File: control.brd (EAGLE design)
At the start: 165 x 34 mm, 65 parts, among them IC3 ATTINY85-20S

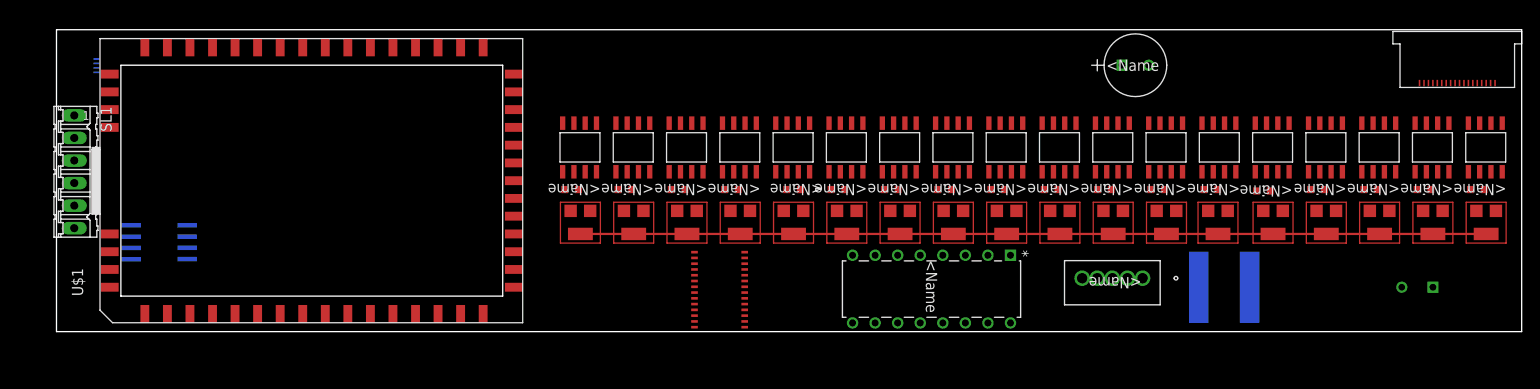
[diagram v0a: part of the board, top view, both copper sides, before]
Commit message: FAIL compact layout
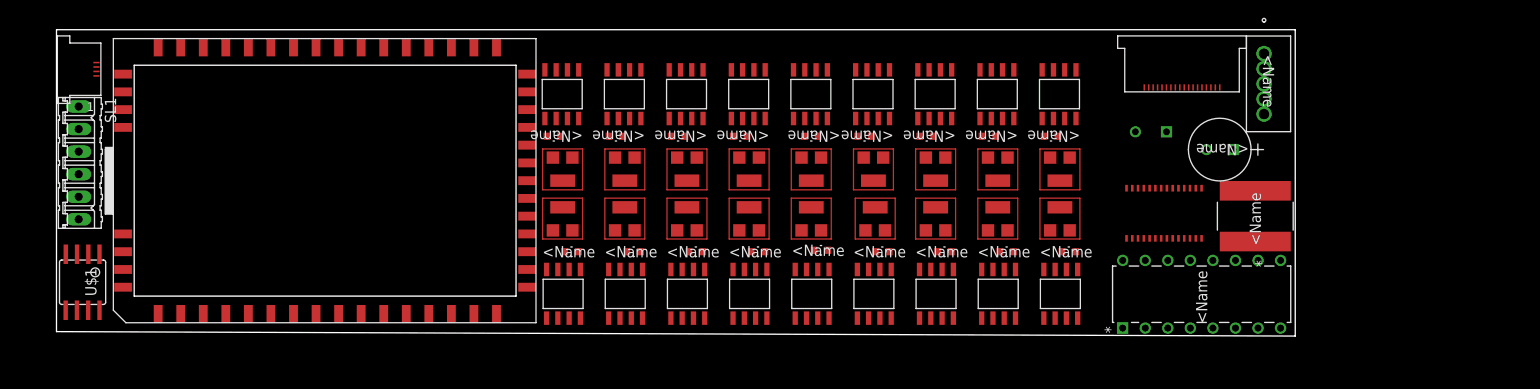
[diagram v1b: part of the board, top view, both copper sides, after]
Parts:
- moved U$18 104.0 mm to (57.0, 14.0), turned to 180 degrees
- moved R8 102.2 mm to (58.0, 9.00), turned to 0 degrees
- moved U$17 100.6 mm to (59.0, 7.00), turned to 180 degrees
- moved U$4 91.0 mm to (64.0, 14.0), turned to 180 degrees
- moved R1 89.3 mm to (65.0, 9.00), turned to 0 degrees
- moved U$3 87.7 mm to (66.0, 7.00), turned to 180 degrees
- moved U$6 78.1 mm to (71.0, 14.0), turned to 180 degrees
- moved R2 76.3 mm to (72.0, 9.00), turned to 0 degrees
- moved U$5 74.8 mm to (73.0, 7.00), turned to 180 degrees
- moved U$8 65.1 mm to (78.0, 14.0), turned to 180 degrees
- moved R3 63.4 mm to (79.0, 9.00), turned to 0 degrees
- moved U$7 62.0 mm to (80.0, 7.00), turned to 180 degrees
- moved U$14 52.1 mm to (85.0, 14.0), turned to 180 degrees
- moved R6 50.3 mm to (86.1, 9.16), turned to 0 degrees
- moved U$13 49.2 mm to (87.0, 7.00), turned to 180 degrees
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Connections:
- removed net B0: IC3.5, SL1.5
- removed net B1: IC3.6, SL1.6
- removed net B2: IC3.7
- removed net N$39: SL1.3
- new net ENC1: IC3.6, SL1.5
- new net ENC2: IC3.7, SL1.6
- new net ENCOUT: IC3.5, U$1.USB1_N
- net 3V3: now also SL1.3
- net LEDSTR_1: now also U$44.P$9; no longer U$44.P$1
- net LEDSTR_11: now also U$44.P$1; no longer U$44.P$9
- net LEDSTR_2: now also U$44.P$8; no longer U$44.P$2
- net LEDSTR_3: now also U$44.P$7; no longer U$44.P$3
- net LEDSTR_4: now also U$44.P$6; no longer U$44.P$4
- net LEDSTR_5: now also U$44.P$3; no longer U$44.P$7
- net LEDSTR_6: now also U$44.P$4; no longer U$44.P$6
- net LEDSTR_8: now also U$44.P$2; no longer U$44.P$8
- net ZN0: now also U$37.P$13; no longer U$37.P$6
- net ZN1: now also U$37.P$12; no longer U$37.P$7
- net ZN2: now also U$37.P$11; no longer U$37.P$8
- net ZN3: now also U$37.P$10; no longer U$37.P$9
- net ZN4: now also U$37.P$9; no longer U$37.P$10
- net ZN5: now also U$37.P$8; no longer U$37.P$11
- net ZN6: now also U$37.P$7; no longer U$37.P$12
- net ZN7: now also U$37.P$6; no longer U$37.P$13
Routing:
- net GND: track 103.0 -> 0.00 mm
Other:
- board size 165 x 34 mm -> 139.5 x 34.5 mm

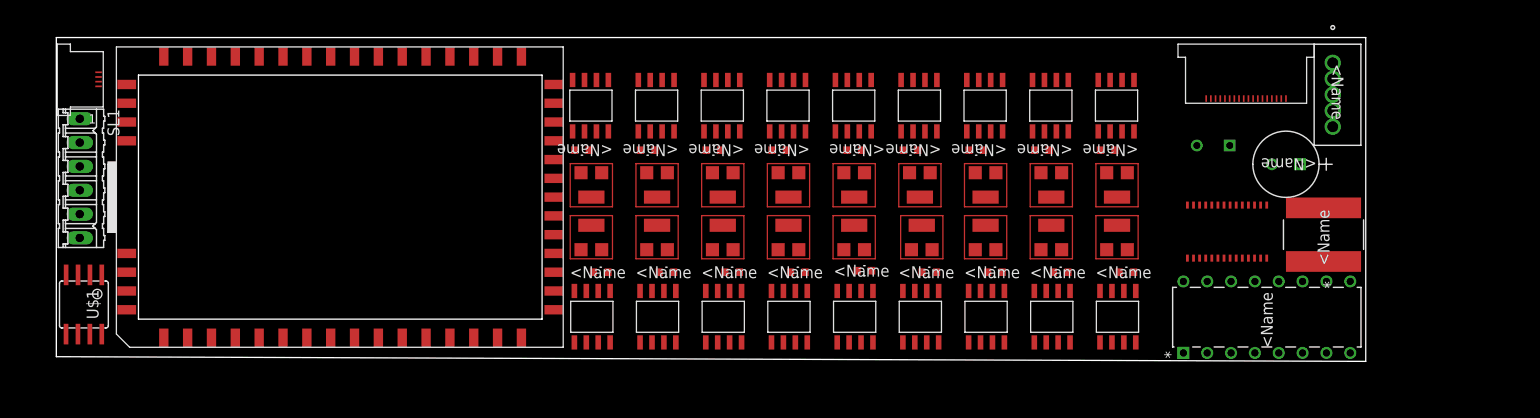
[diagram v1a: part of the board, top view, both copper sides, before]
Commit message: completes first ideration
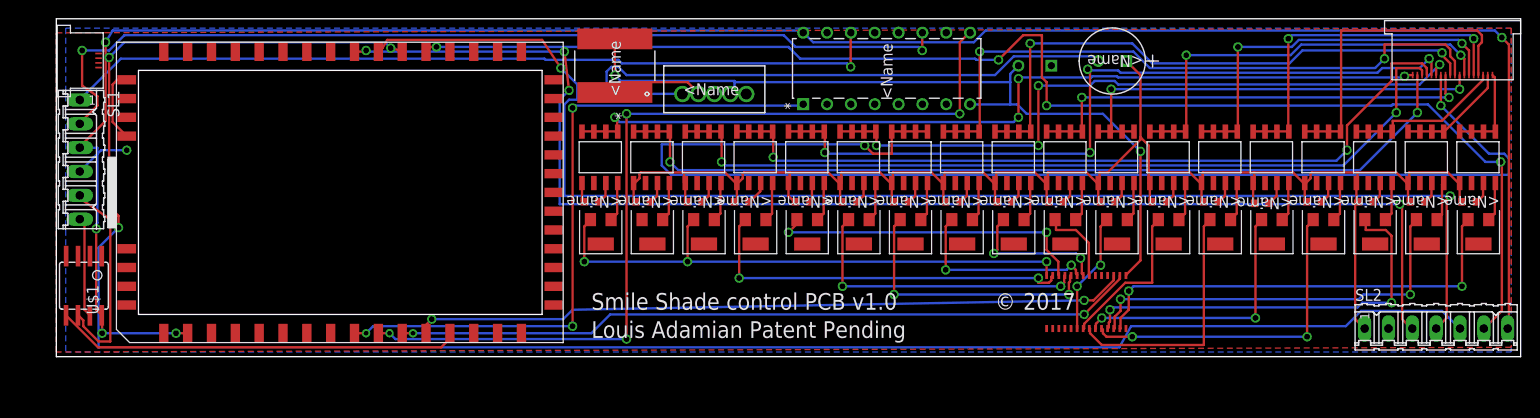
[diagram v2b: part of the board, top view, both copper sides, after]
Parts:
- removed U$43: 2N7002P, LED Driver:SOT23
- added SL2: (no value), con-amp-quick:07P
- added U$38: 2N7002P, Smile_Shade:SOT23
- U$10, U$12, U$14, U$16, U$18, U$20, U$22, U$24, U$26, U$28, U$30, U$32, U$34, U$4, U$41, U$6, U$8: device LED Driver:SOT23 -> Smile_Shade:SOT23
- moved R8 92.8 mm to (150.5, 16.5), turned to 180 degrees
- moved U$17 91.2 mm to (149.5, 18.5), turned to 0 degrees
- moved U$4 82.0 mm to (146.0, 12.0), turned to 0 degrees
- moved R1 80.4 mm to (145.0, 16.5), turned to 180 degrees
- moved U$3 78.8 mm to (144.0, 18.5), turned to 0 degrees
- moved U$36 77.6 mm to (59.5, 31.0)
- moved U$6 69.5 mm to (140.5, 12.0), turned to 0 degrees
- moved R2 67.9 mm to (139.5, 16.5), turned to 180 degrees
- moved U$5 66.5 mm to (138.5, 18.5), turned to 0 degrees
- moved U$35 63.7 mm to (73.5, 29.0), turned to 0 degrees
- moved U$8 57.0 mm to (135.0, 12.0), turned to 0 degrees
- moved R3 55.5 mm to (134.0, 16.5), turned to 180 degrees
- moved U$7 54.2 mm to (133.0, 18.5), turned to 0 degrees
- moved U$2 48.4 mm to (97.3, 34.5)
- moved R6 42.9 mm to (128.4, 16.3), turned to 180 degrees
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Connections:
- removed net 24V: U$2.8
- new net +3V3: IC3.8
- new net ENDSTOP0: SL2.3, U$1.CSID0
- new net ENDSTOP1: SL2.4, U$1.CSID1
- new net ENDSTOP2: SL2.5, U$1.CSID2
- new net ENDSTOP3: SL2.6, U$1.CSID3
- net 3V3: now also SL2.7, U$2.16; no longer IC3.8
- net 48V: now also SL2.1
- net 5V: now also U$2.8; no longer U$2.16
- net ENCOUT: now also U$1.UART2-TX; no longer U$1.USB1_N
- net GND: now also SL2.2, U$38.P$1; no longer U$43.P$1
- net LEDSTR_1: now also U$44.P$1; no longer U$44.P$9
- net LEDSTR_11: now also U$44.P$11; no longer U$44.P$1
- net LEDSTR_2: now also U$44.P$2; no longer U$44.P$8
- net LEDSTR_3: now also U$44.P$3; no longer U$44.P$7
- net LEDSTR_4: now also U$44.P$4; no longer U$44.P$6
- net LEDSTR_5: now also U$44.P$7; no longer U$44.P$3
- net LEDSTR_6: now also U$44.P$6; no longer U$44.P$4
- net LEDSTR_8: now also U$44.P$8; no longer U$44.P$2
- net LEDSTR_9: now also U$44.P$9; no longer U$44.P$11
- net N$11: now also U$12.P$3; no longer U$14.P$3
- net N$13: now also U$10.P$3; no longer U$16.P$3
- net N$15: now also U$38.P$3; no longer U$18.P$3
- net N$17: now also U$18.P$3; no longer U$20.P$3
- net N$19: now also U$20.P$3; no longer U$22.P$3
- net N$21: now also U$22.P$3; no longer U$24.P$3
- net N$23: now also U$24.P$3; no longer U$26.P$3
- net N$25: now also U$32.P$3; no longer U$28.P$3
- net N$29: now also U$28.P$3; no longer U$32.P$3
- net N$31: now also U$26.P$3; no longer U$34.P$3
- net N$35: now also U$34.P$3; no longer U$41.P$3
- net N$37: now also U$41.P$3; no longer U$43.P$3
- net N$7: now also U$16.P$3; no longer U$10.P$3
- net N$9: now also U$14.P$3; no longer U$12.P$3
- net ZN0: now also U$38.P$2; no longer U$18.P$2
- net ZN11: now also U$32.P$2; no longer U$28.P$2
- net ZN12: now also U$24.P$2; no longer U$26.P$2
- net ZN13: now also U$18.P$2; no longer U$20.P$2
- net ZN14: now also U$20.P$2; no longer U$22.P$2
- net ZN15: now also U$22.P$2; no longer U$24.P$2
- net ZN16: now also U$41.P$2; no longer U$43.P$2
- net ZN4: now also U$12.P$2; no longer U$14.P$2
- net ZN5: now also U$14.P$2; no longer U$12.P$2
- net ZN6: now also U$16.P$2; no longer U$10.P$2
- net ZN7: now also U$10.P$2; no longer U$16.P$2
- net ZN8: now also U$26.P$2; no longer U$41.P$2
- net ZN9: now also U$28.P$2; no longer U$32.P$2
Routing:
- net 3V3: track 0.00 -> 225.4 mm, vias 0 -> 5
- net ENDSTOP2: track 0.00 -> 212.2 mm, vias 0 -> 3
- net 48V: track 0.00 -> 175.5 mm
- net ENDSTOP1: track 0.00 -> 146.3 mm, vias 0 -> 2
- net ENDSTOP3: track 0.00 -> 144.8 mm, vias 0 -> 4
- net ENDSTOP0: track 0.00 -> 142.6 mm, vias 0 -> 4
- net LEDSTR_12: track 0.00 -> 138.6 mm, vias 0 -> 2
- net M2B: track 0.00 -> 102.2 mm, vias 0 -> 2
- net LEDSTR_17: track 0.00 -> 95.4 mm, vias 0 -> 4
- net M1: track 0.00 -> 95.3 mm, vias 0 -> 4
- net LEDSTR_18: track 0.00 -> 93.6 mm, vias 0 -> 2
- net LEDSTR_16: track 0.00 -> 89.6 mm, vias 0 -> 2
- net M2A: track 0.00 -> 88.0 mm, vias 0 -> 1
- net 5V: track 0.00 -> 86.4 mm, vias 0 -> 2
- net LEDSTR_15: track 0.00 -> 84.3 mm, vias 0 -> 2
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- added copper zone on layer 16, net 48V
- added copper zone on layer 1, net GND
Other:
- board size 139.5 x 34.5 mm -> 156 x 36 mm
- board text added: "2017"
- board text added: "Louis Adamian Patent Pending"
- board text added: "Smile Shade control PCB v1.0"
- board text added: "©"

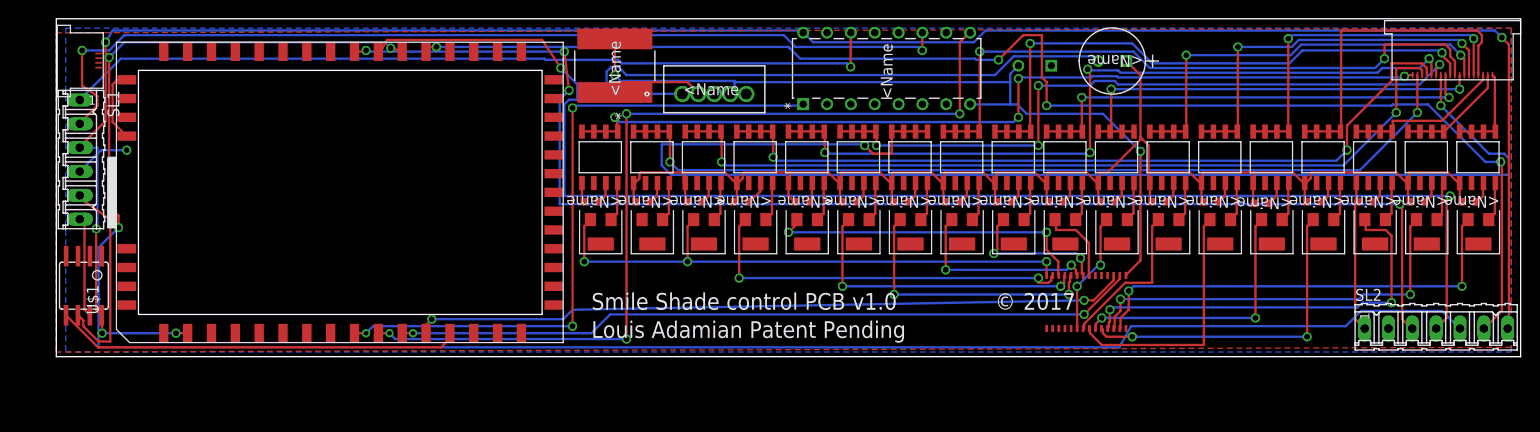
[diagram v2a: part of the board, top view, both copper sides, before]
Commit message: adds actual route
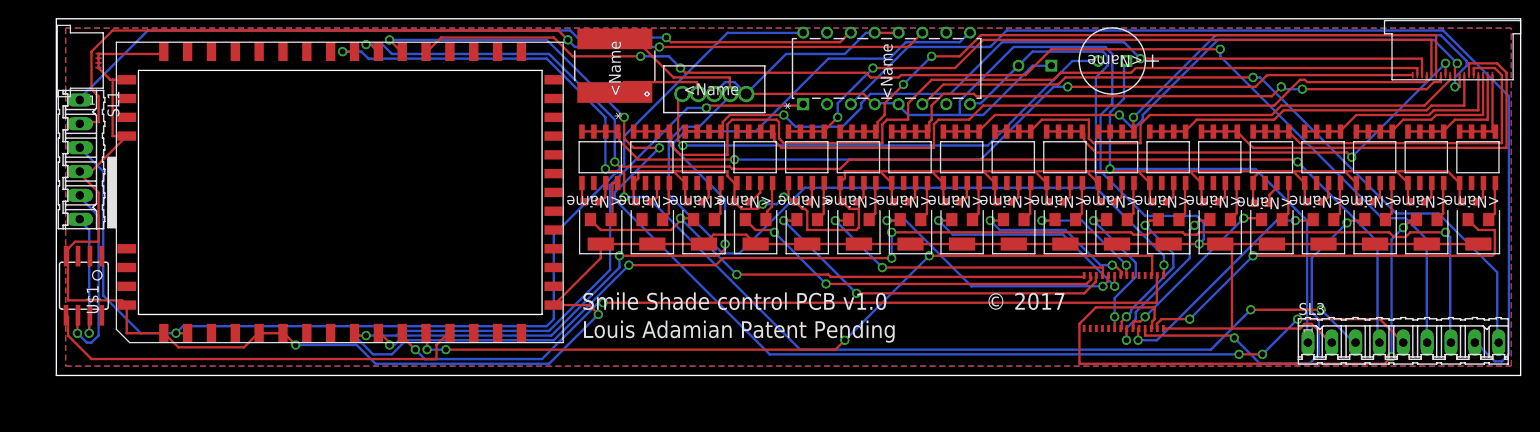
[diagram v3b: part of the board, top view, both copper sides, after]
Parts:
- removed SL2: (no value), con-amp-quick:07P
- added SL3: (no value), con-amp-quick:09P
- moved U$37 4.00 mm to (109.5, 3.00)
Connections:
- net 3V3: now also SL3.7; no longer SL2.7
- net 48V: now also SL3.1; no longer SL2.1
- net ENDSTOP0: now also SL3.3; no longer SL2.3
- net ENDSTOP1: now also SL3.4; no longer SL2.4
- net ENDSTOP2: now also SL3.5; no longer SL2.5
- net ENDSTOP3: now also SL3.6; no longer SL2.6
- net GND: now also SL3.2; no longer SL2.2
- net M1A: now also SL3.8
- net M1B: now also SL3.9
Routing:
- net GND: track 13.8 -> 352.8 mm, vias 1 -> 3
- net M1A: track 0.00 -> 108.5 mm
- net M1B: track 0.00 -> 78.6 mm, vias 0 -> 1
- net LEDSTR_12: track 138.6 -> 63.3 mm
- net ENDSTOP2: track 212.2 -> 137.6 mm, vias 3 -> 6
- net 5V: track 86.4 -> 125.6 mm, vias 2 -> 1
- net 48V: track 175.5 -> 208.0 mm, vias 0 -> 3
- net 3V3: track 225.4 -> 252.4 mm
- net ZN1: track 42.8 -> 65.0 mm
- net ENDSTOP3: track 144.8 -> 130.1 mm, vias 4 -> 3
- net ENDSTOP1: track 146.3 -> 132.5 mm, vias 2 -> 3
- net ENDSTOP0: track 142.6 -> 130.2 mm, vias 4 -> 5
- net LEDSTR_4: track 34.3 -> 23.3 mm
- net N$34: track 64.4 -> 54.0 mm, vias 0 -> 1
- net ZN3: track 35.2 -> 25.3 mm
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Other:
- board size 156 x 36 mm -> 156 x 38 mm
